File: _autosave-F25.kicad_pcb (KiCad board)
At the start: 2 copper layers, 45 x 30 mm, 44 parts, among them J3 B2B-PH-K-S, J4 USB_C_Receptacle_USB2.0_16P, Q1 IRLML6244, SW1 RESET, SW2 BOOT, U1 MS5611-01BA, U2 MPU-6050, U4 ESP32-S3-WROOM-1-N8, U5 AP2112K-3.3

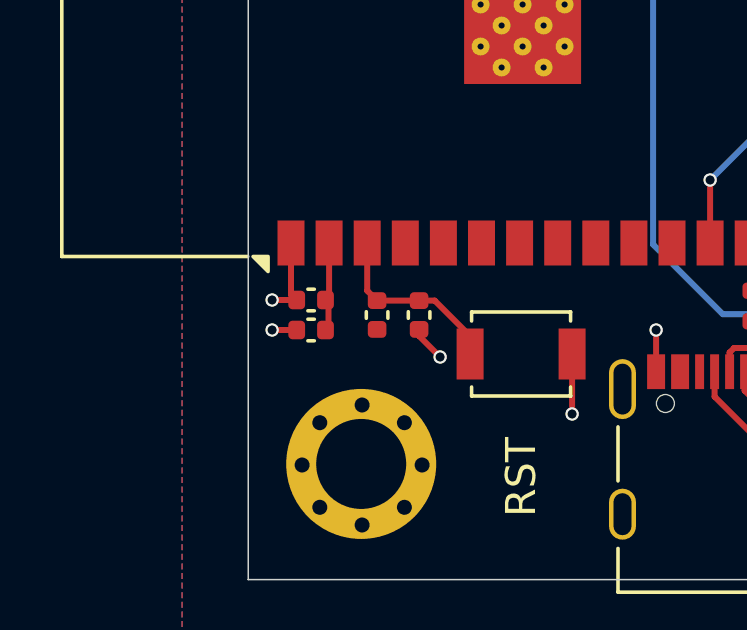
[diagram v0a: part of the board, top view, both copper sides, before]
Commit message: Updates to Name
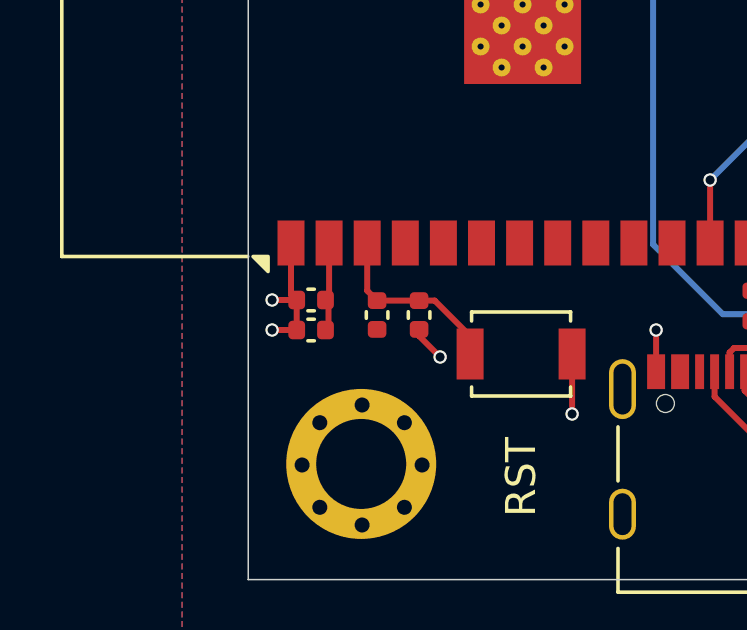
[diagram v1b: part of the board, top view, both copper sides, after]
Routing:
- net BAT-: track 34.9 -> 35.9 mm
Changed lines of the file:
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@@
 			)
 		)
-		(property "LCSC" "C2286"
+		(property "LCSC" "C2290"
 			(at 0 0 180)
 			(unlocked yes)
@@
 			)
 		)
-		(property "LCSC" "C2290"
+		(property "LCSC" "C2288"
 			(at 0 0 180)
 			(unlocked yes)
@@
 		(width 0.2)
 		(layer "F.Cu")
+		(net 5)
+	)
+	(segment
+		(start 137.32 106)
+		(end 137.32 107)
+		(width 0.2)
+		(layer "F.Cu")
